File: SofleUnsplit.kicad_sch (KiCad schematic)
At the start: 117 parts, among them SW1 Switch, SW10 Switch, SW11 Switch, SW12 Switch, SW13 Switch, SW14 Switch, SW15 Switch, SW16 Switch, SW17 Switch, SW18 Switch, SW19 Switch, SW2 Switch, SW20 Switch, SW21 Switch, SW22 Switch, SW23 Switch, SW24 Switch, SW25 Switch, SW26 Switch, SW27 Switch, SW28 Switch, SW29 Switch, SW3 Switch, SW30 Switch, SW31 Switch, SW32 Switch, SW33 Switch, SW34 Switch, SW35 Switch, SW36 Switch, SW37 Switch, SW38 Switch, SW39 Switch, SW4 Switch, SW40 Switch, SW41 Switch, SW42 Switch, SW43 Switch, SW44 Switch, SW45 Switch, SW46 Switch, SW47 Switch, SW48 Switch, SW49 Switch, SW5 Switch, SW50 Switch, SW51 Switch, SW52 Switch, SW53 Switch, SW54 Switch, SW55 Switch, SW56 Switch, SW57 Switch, SW58 Switch, SW6 Switch, SW7 Switch, SW8 Switch, SW9 Switch, U1 MCU_rp2040-zero

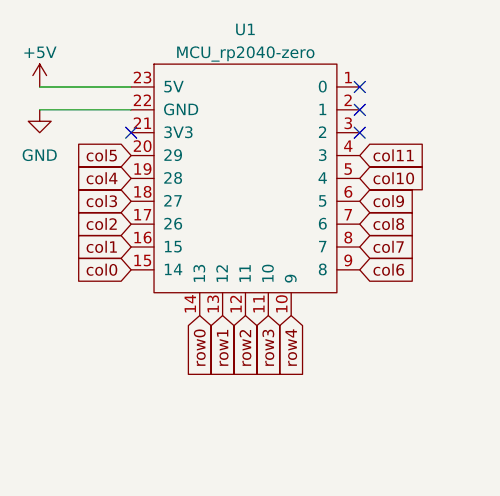
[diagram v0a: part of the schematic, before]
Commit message: Routing done
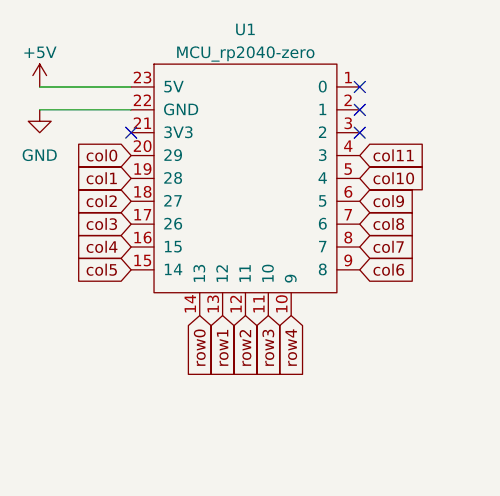
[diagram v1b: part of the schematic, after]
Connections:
- net col0: now also U1.20 (29); no longer U1.15 (14)
- net col1: now also U1.19 (28); no longer U1.16 (15)
- net col2: now also U1.18 (27); no longer U1.17 (26)
- net col3: now also U1.17 (26); no longer U1.18 (27)
- net col4: now also U1.16 (15); no longer U1.19 (28)
- net col5: now also U1.15 (14); no longer U1.20 (29)
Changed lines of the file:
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@@
     )
   )
-  (global_label "col4" (shape input) (at 40.64 53.34 180) (fields_autoplaced)
+  (global_label "col4" (shape input) (at 40.64 60.96 180) (fields_autoplaced)
     (effects (font (size 1.27 1.27)) (justify right))
-    (property "Intersheetrefs" "${INTERSHEET_REFS}" (at 33.6219 53.34 0)
+    (property "Intersheetrefs" "${INTERSHEET_REFS}" (at 33.6219 60.96 0)
       (effects (font (size 1.27 1.27)) (justify right) hide)
     )
@@
     )
   )
-  (global_label "col2" (shape input) (at 40.64 58.42 180) (fields_autoplaced)
+  (global_label "col2" (shape input) (at 40.64 55.88 180) (fields_autoplaced)
+    (effects (font (size 1.27 1.27)) (justify right))
+    (property "Intersheetrefs" "${INTERSHEET_REFS}" (at 33.6219 55.88 0)
+      (effects (font (size 1.27 1.27)) (justify right) hide)
+    )
+  )
+  (global_label "col3" (shape input) (at 40.64 58.42 180) (fields_autoplaced)
     (effects (font (size 1.27 1.27)) (justify right))
     (property "Intersheetrefs" "${INTERSHEET_REFS}" (at 33.6219 58.42 0)
@@
     )
   )
-  (global_label "col3" (shape input) (at 40.64 55.88 180) (fields_autoplaced)
+  (global_label "col1" (shape input) (at 40.64 53.34 180) (fields_autoplaced)
     (effects (font (size 1.27 1.27)) (justify right))
-    (property "Intersheetrefs" "${INTERSHEET_REFS}" (at 33.6219 55.88 0)
-      (effects (font (size 1.27 1.27)) (justify right) hide)
-    )
-  )
-  (global_label "col1" (shape input) (at 40.64 60.96 180) (fields_autoplaced)
-    (effects (font (size 1.27 1.27)) (justify right))
-    (property "Intersheetrefs" "${INTERSHEET_REFS}" (at 33.6219 60.96 0)
+    (property "Intersheetrefs" "${INTERSHEET_REFS}" (at 33.6219 53.34 0)
       (effects (font (size 1.27 1.27)) (justify right) hide)
     )
@@
     )
   )
-  (global_label "col0" (shape input) (at 40.64 63.5 180) (fields_autoplaced)
+  (global_label "col0" (shape input) (at 40.64 50.8 180) (fields_autoplaced)
+    (effects (font (size 1.27 1.27)) (justify right))
+    (property "Intersheetrefs" "${INTERSHEET_REFS}" (at 33.6219 50.8 0)
+      (effects (font (size 1.27 1.27)) (justify right) hide)
+    )
+  )
+  (global_label "col5" (shape input) (at 40.64 63.5 180) (fields_autoplaced)
     (effects (font (size 1.27 1.27)) (justify right))
     (property "Intersheetrefs" "${INTERSHEET_REFS}" (at 33.6219 63.5 0)
       (effects (font (size 1.27 1.27)) (justify right) hide)
     )
-  )
-  (global_label "col5" (shape input) (at 40.64 50.8 180) (fields_autoplaced)
-    (effects (font (size 1.27 1.27)) (justify right))
-    (property "Intersheetrefs" "${INTERSHEET_REFS}" (at 33.6219 50.8 0)
-      (effects (font (size 1.27 1.27)) (justify right) hide)
-    )

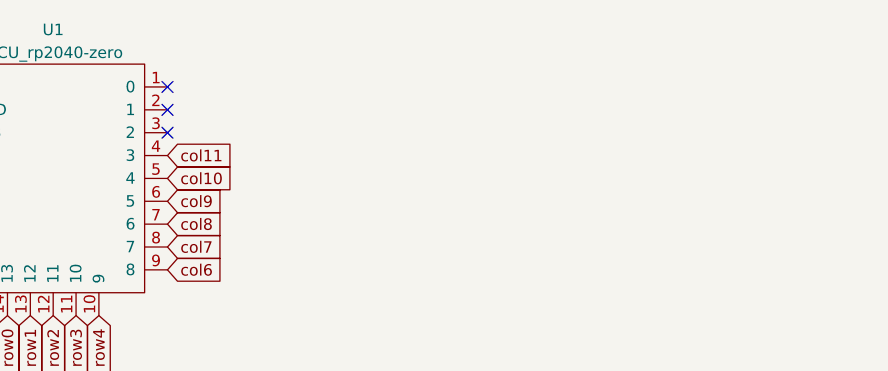
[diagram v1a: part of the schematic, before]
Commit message: Polishing, finishing
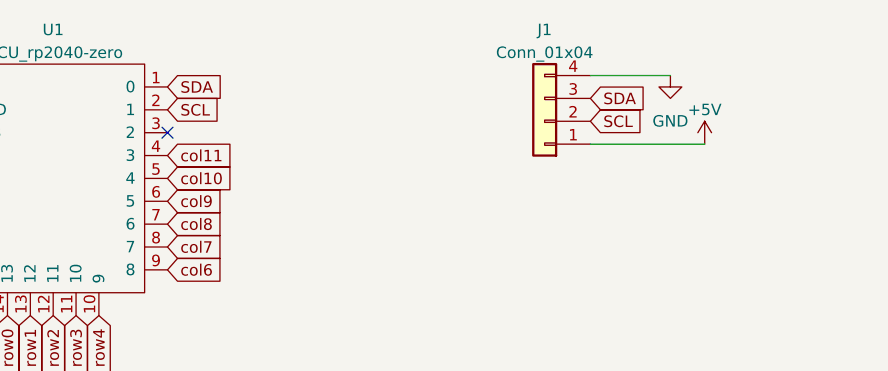
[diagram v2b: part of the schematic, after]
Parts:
- added J1: Conn_01x04, Connector_PinSocket_2.54mm:PinSocket_1x04_P2.54mm_Vertical, symbol Connector_Generic:Conn_01x04
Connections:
- net +5V: now also J1.1 (Pin_1)
- net GND: now also J1.4 (Pin_4)
- net SDA: now reaches U1.1 (0)
- net SDA: now also J1.3 (Pin_3)
- net SCL: now reaches U1.2 (1)
- net SCL: now also J1.2 (Pin_2)
- no-connect marks 4 -> 2
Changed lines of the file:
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@@
   (junction (at 326.39 191.77) (diameter 0) (color 0 0 0 0)
   )
-  (no_connect (at 66.04 43.18))
   (no_connect (at 40.64 48.26))
   (no_connect (at 66.04 48.26))
-  (no_connect (at 66.04 45.72))
   (wire (pts (xy 43.18 208.28) (xy 67.31 208.28))
     (stroke (width 0) (type default))
@@
     (stroke (width 0) (type default))
   )
+  (wire (pts (xy 113.03 41.91) (xy 121.92 41.91))
+    (stroke (width 0) (type default))
+  )
   (wire (pts (xy 96.52 208.28) (xy 124.46 208.28))
     (stroke (width 0) (type default))
@@
     (stroke (width 0) (type default))
   )
+  (wire (pts (xy 113.03 49.53) (xy 125.73 49.53))
+    (stroke (width 0) (type default))
+  )
   (wire (pts (xy 251.46 167.64) (xy 251.46 184.15))
     (stroke (width 0) (type default))
@@
     )
   )
+  (global_label "SCL" (shape input) (at 66.04 45.72 0) (fields_autoplaced)
+    (effects (font (size 1.27 1.27)) (justify left))
+    (property "Intersheetrefs" "${INTERSHEET_REFS}" (at 72.4534 45.72 0)
+      (effects (font (size 1.27 1.27)) (justify left) hide)
+    )
+  )
   (global_label "col4" (shape input) (at 166.37 157.48 90) (fields_autoplaced)
     (effects (font (size 1.27 1.27)) (justify left))
@@
     )
   )
+  (global_label "SDA" (shape input) (at 66.04 43.18 0) (fields_autoplaced)
+    (effects (font (size 1.27 1.27)) (justify left))
+    (property "Intersheetrefs" "${INTERSHEET_REFS}" (at 72.5139 43.18 0)
+      (effects (font (size 1.27 1.27)) (justify left) hide)
+    )
+  )
   (global_label "col5" (shape input) (at 195.58 157.48 90) (fields_autoplaced)
     (effects (font (size 1.27 1.27)) (justify left))
@@
     )
   )
+  (global_label "SDA" (shape input) (at 113.03 44.45 0) (fields_autoplaced)
+    (effects (font (size 1.27 1.27)) (justify left))
+    (property "Intersheetrefs" "${INTERSHEET_REFS}" (at 119.5039 44.45 0)
+      (effects (font (size 1.27 1.27)) (justify left) hide)
+    )
+  )
+  (global_label "SCL" (shape input) (at 113.03 46.99 0) (fields_autoplaced)
+    (effects (font (size 1.27 1.27)) (justify left))
+    (property "Intersheetrefs" "${INTERSHEET_REFS}" (at 119.4434 46.99 0)
+      (effects (font (size 1.27 1.27)) (justify left) hide)
+    )
+  )
   (global_label "col1" (shape input) (at 81.28 157.48 90) (fields_autoplaced)
     (effects (font (size 1.27 1.27)) (justify left))
@@
     )
   )
+  (symbol (lib_id "power:+5V") (at 125.73 49.53 0) (unit 1)
+    (in_bom yes) (on_board yes) (dnp no) (fields_autoplaced)
+    (property "Reference" "#PWR03" (at 125.73 53.34 0)
+      (effects (font (size 1.27 1.27)) hide)
+    )
+    (property "Value" "+5V" (at 125.73 45.72 0)
+      (effects (font (size 1.27 1.27)))
+    )
+    (property "Footprint" "" (at 125.73 49.53 0)
+      (effects (font (size 1.27 1.27)) hide)
+    )
+    (property "Datasheet" "" (at 125.73 49.53 0)
+      (effects (font (size 1.27 1.27)) hide)
+    )
+    (pin "1")
+    (instances
+      (project "SofleUnsplit"
+        (path "/0271784e-2195-481b-b0c9-914478a67f87"
+          (reference "#PWR03") (unit 1)
+        )
+      )
+    )
+  )
   (symbol (lib_id "Diode:1N4148W") (at 326.39 220.98 90) (unit 1)
     (in_bom yes) (on_board yes) (dnp no) (fields_autoplaced)
@@
     )
   )
+  (symbol (lib_id "Connector_Generic:Conn_01x04") (at 107.95 46.99 180) (unit 1)
+    (in_bom yes) (on_board yes) (dnp no) (fields_autoplaced)
+    (property "Reference" "J1" (at 107.95 36.83 0)
+      (effects (font (size 1.27 1.27)))
+    )
+    (property "Value" "Conn_01x04" (at 107.95 39.37 0)
+      (effects (font (size 1.27 1.27)))
+    )
+    (property "Footprint" "Connector_PinSocket_2.54mm:PinSocket_1x04_P2.54mm_Vertical" (at 107.95 46.99 0)
+      (effects (font (size 1.27 1.27)) hide)
+    )
+    (property "Datasheet" "~" (at 107.95 46.99 0)
+      (effects (font (size 1.27 1.27)) hide)
+    )
+    (pin "1")
+    (pin "2")
+    (pin "3")
+    (pin "4")
+    (instances
+      (project "SofleUnsplit"
+        (path "/0271784e-2195-481b-b0c9-914478a67f87"
+          (reference "J1") (unit 1)
+        )
+      )
+    )
+  )
   (symbol (lib_id "zzkeeb:Switch") (at 144.78 200.66 0) (unit 1)
     (in_bom yes) (on_board yes) (dnp no)
@@
         )
       )
+    )
+  )
+  (symbol (lib_id "power:GND") (at 121.92 41.91 0) (unit 1)
+    (in_bom yes) (on_board yes) (dnp no) (fields_autoplaced)
+    (property "Reference" "#PWR04" (at 121.92 48.26 0)
+      (effects (font (size 1.27 1.27)) hide)
+    )
+    (property "Value" "GND" (at 121.92 46.99 0)
+      (effects (font (size 1.27 1.27)))
+    )
+    (property "Footprint" "" (at 121.92 41.91 0)
+      (effects (font (size 1.27 1.27)) hide)
+    )
+    (property "Datasheet" "" (at 121.92 41.91 0)
+      (effects (font (size 1.27 1.27)) hide)
+    )
+    (pin "1")
+    (instances
+      (project "SofleUnsplit"
+        (path "/0271784e-2195-481b-b0c9-914478a67f87"
+          (reference "#PWR04") (unit 1)
+        )
+      )

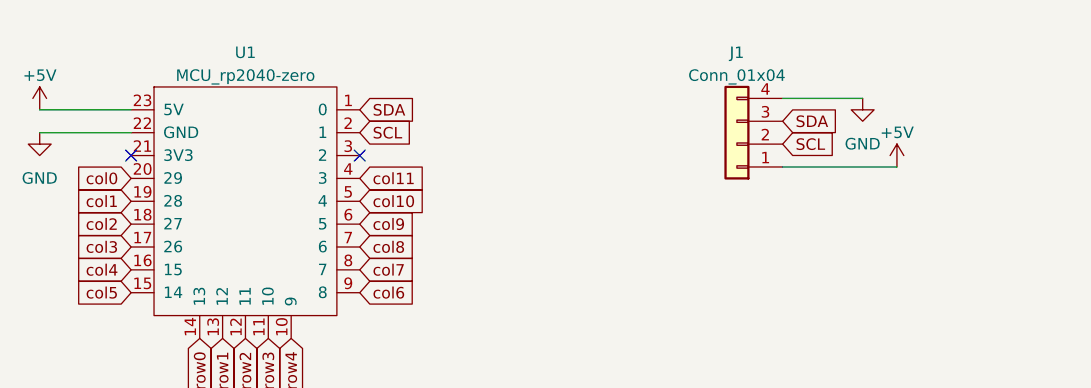
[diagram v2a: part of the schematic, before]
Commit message: Finalising
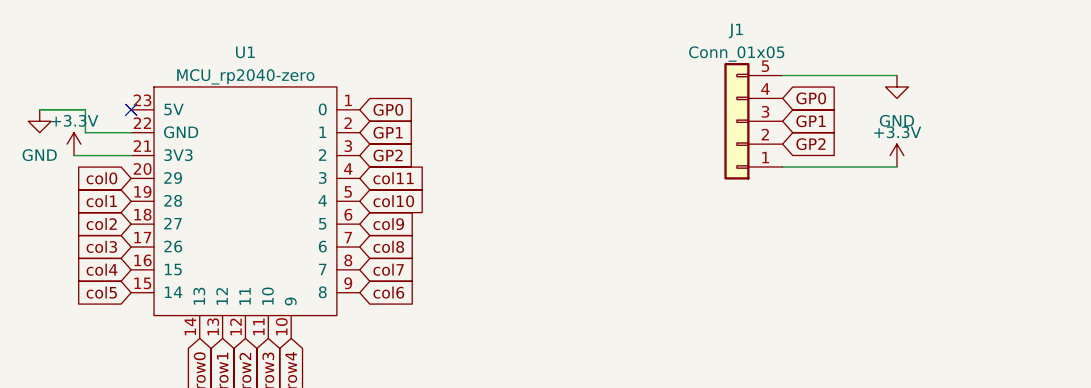
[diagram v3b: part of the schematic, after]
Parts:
- removed J1: Conn_01x04, Connector_PinSocket_2.54mm:PinSocket_1x04_P2.54mm_Vertical, symbol Connector_Generic:Conn_01x04
- added J1: Conn_01x05, Connector_PinSocket_2.54mm:PinSocket_1x05_P2.54mm_Vertical, symbol Connector_Generic:Conn_01x05
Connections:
- net GND: now also J1.5 (Pin_5)
- net +3.3V: now reaches U1.21 (3V3)
- net +3.3V: now also J1.1 (Pin_1)
- net GP2: now reaches U1.3 (2)
- net GP2: now also J1.2 (Pin_2)
- net +5V: no longer names the net of U1.23 (5V)
- net SCL renamed GP1
- net GP1: now also J1.3 (Pin_3)
- net SDA renamed GP0
- net GP0: now also J1.4 (Pin_4)
- no-connect marks 2 -> 1
